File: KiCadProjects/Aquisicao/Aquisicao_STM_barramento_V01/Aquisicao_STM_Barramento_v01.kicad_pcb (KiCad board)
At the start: 2 copper layers, 90 x 100 mm, 3 parts, among them J1 alimentacao analogica, J2 sinais analogicos, J3 comunicacao / sinais digitais

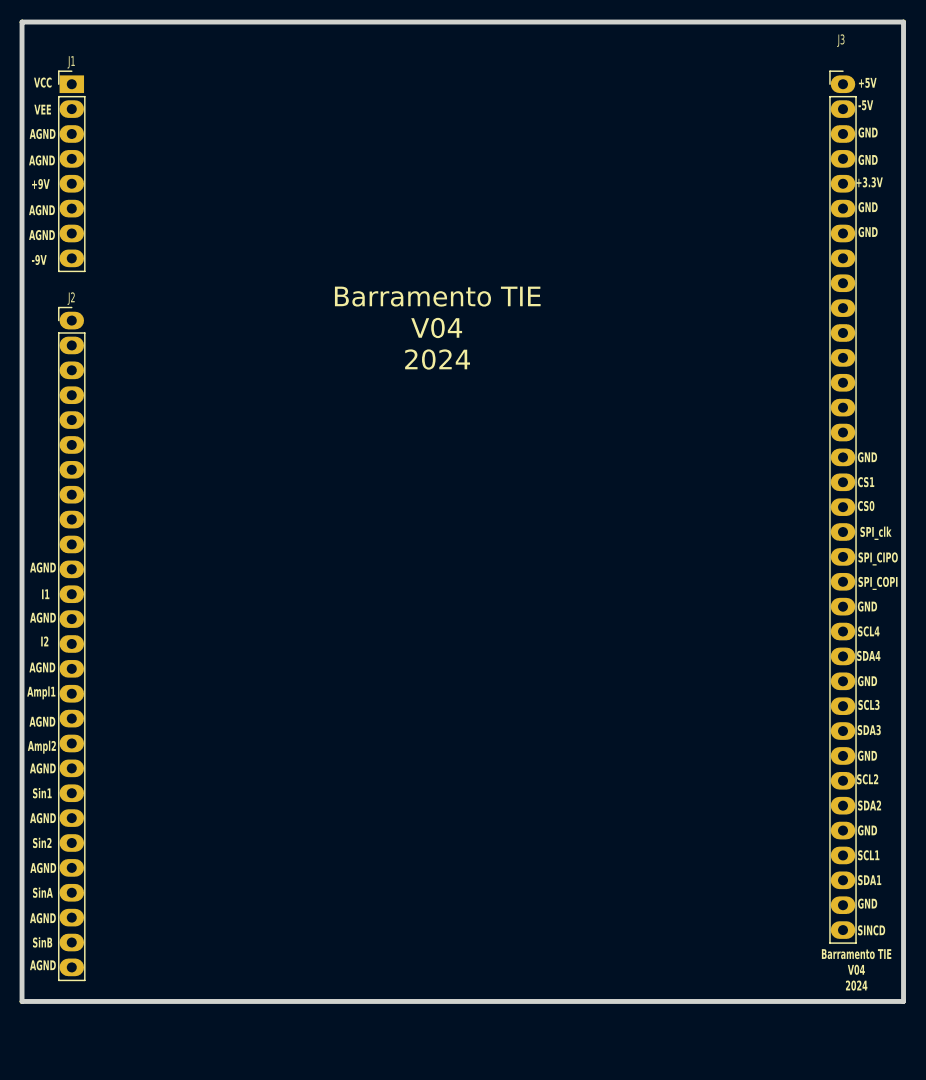
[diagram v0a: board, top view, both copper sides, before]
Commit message: tmp
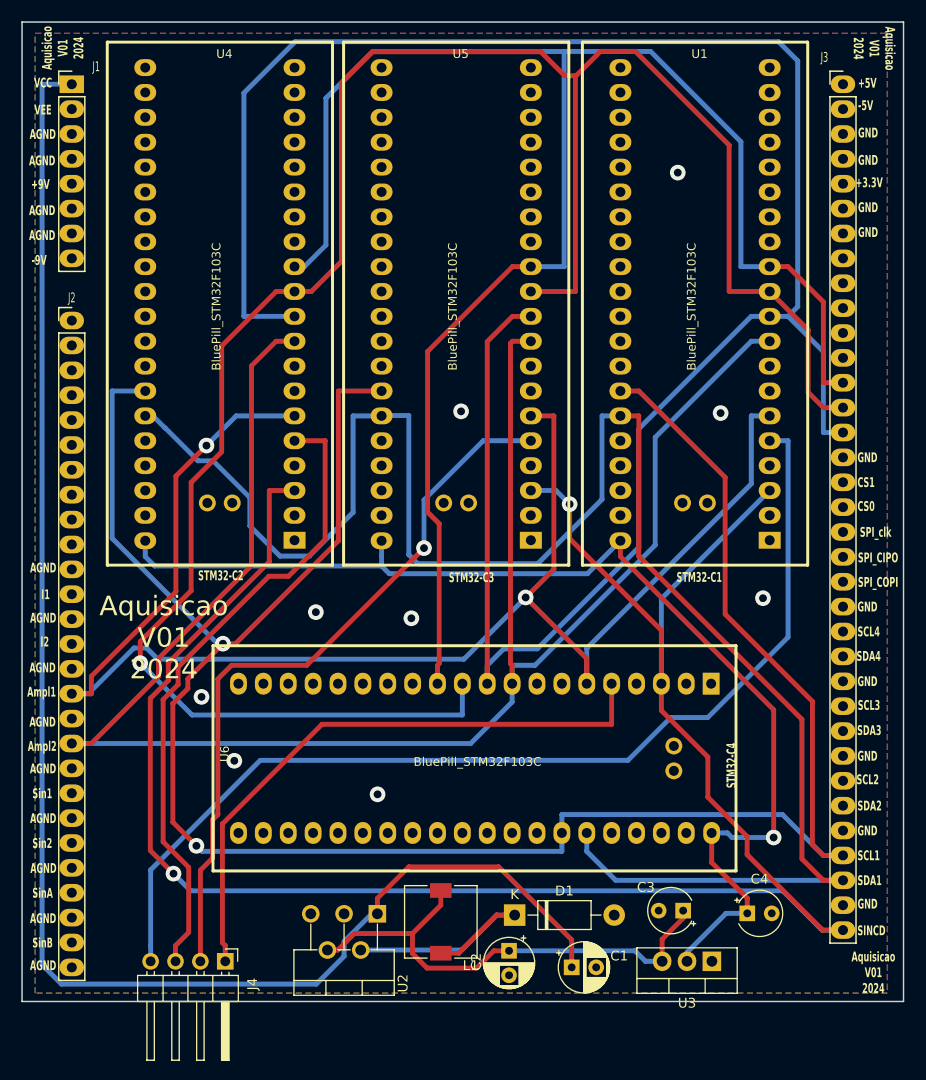
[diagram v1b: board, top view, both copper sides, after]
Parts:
- added C1: 680u, Capacitor_THT:CP_Radial_D5.0mm_P2.50mm, F.Cu at (157.7, 147.3)
- added C2: 220u, Capacitor_THT:CP_Radial_D5.0mm_P2.50mm, F.Cu at (151.3, 145.6)
- added C3: 10uF, Capacitor_THT:CP_Radial_Tantal_D4.5mm_P2.50mm, F.Cu at (169.1, 141.5)
- added C4: 33uF, Capacitor_THT:CP_Radial_Tantal_D4.5mm_P2.50mm, F.Cu at (175.6, 141.8)
- added D1: 1N5819, Diode_THT:D_DO-41_SOD81_P10.16mm_Horizontal, F.Cu at (151.9, 142.0)
- added J4: Conn_01x04, Connector_PinHeader_2.54mm:PinHeader_1x04_P2.54mm_Horizontal, F.Cu at (122.3, 146.7)
- added L1: 33u, Inductor_SMD:L_7.3x7.3_H4.5, F.Cu at (144.4, 142.7)
- added U1: BluePill_STM32F103C, BluePill_STM32:BluePill_STM32F103C, F.Cu at (177.9, 103.7)
- added U2: LM2596S-5, Package_TO_SOT_THT:TO-220-5_P3.4x3.7mm_StaggerOdd_Lead3.8mm_Vertical, F.Cu at (137.9, 141.8)
- added U3: LM1117T-3.3, Package_TO_SOT_THT:TO-220-3_Vertical, F.Cu at (172.0, 146.7)
- added U4: BluePill_STM32F103C, BluePill_STM32:BluePill_STM32F103C, F.Cu at (129.4, 103.7)
- added U5: BluePill_STM32F103C, BluePill_STM32:BluePill_STM32F103C, F.Cu at (153.6, 103.7)
- added U6: BluePill_STM32F103C, BluePill_STM32:BluePill_STM32F103C, F.Cu at (171.9, 118.4)
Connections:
- J3 pad 13: unconnected-(J3-Pin_13-Pad13) -> SINC_C
- J3 pad 14: unconnected-(J3-Pin_14-Pad14) -> SINC_B
- J3 pad 15: unconnected-(J3-Pin_15-Pad15) -> SINC_A
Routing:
- net SCL1: track 0.00 -> 224.6 mm, vias 0 -> 2
- net SINC_A: track 0.00 -> 224.2 mm
- net SINC_B: track 0.00 -> 216.9 mm, vias 0 -> 1
- net SINCD: track 0.00 -> 203.6 mm, vias 0 -> 2
- net Ampl2: track 0.00 -> 186.7 mm
- net SDA1: track 0.00 -> 182.1 mm
- net SINC_C: track 0.00 -> 175.7 mm
- net Ampl1: track 0.00 -> 163.6 mm, vias 0 -> 2
- net VCC: track 0.00 -> 160.5 mm
- net 3.3V_step: track 0.00 -> 116.5 mm, vias 0 -> 1
- net sign_C1: track 0.00 -> 106.2 mm
- net sign_C3: track 0.00 -> 74.5 mm, vias 0 -> 1
- net sign_C2: track 0.00 -> 65.9 mm
- net sign_C4: track 0.00 -> 62.3 mm
- net 5V_stepdown: track 0.00 -> 50.4 mm
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- added copper zone on B.Cu, net Earth
- added copper zone on F.Cu, net Earth
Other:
- board text added: "Aquisicao V01 2024"
- board text added: "STM32-C1"
- board text added: "STM32-C2"
- board text added: "STM32-C3"
- board text added: "STM32-C4"
- board text removed: "Barramento TIE V04 2024"
